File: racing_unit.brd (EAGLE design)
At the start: 81 x 80 mm, 55 parts, among them IC1 78L05Z, IC2 78L05Z, IC3 78L05Z, IC4 78L05Z, J1 J10MM, J2 J10MM, J3 J5MM, J4 J5MM, J5 J7MM, J7 J5MM, J8 J5MM, J9 J5MM, Q1 BDX54C, Q2 BDX54C, Q3 BDX54C, Q4 BDX54C

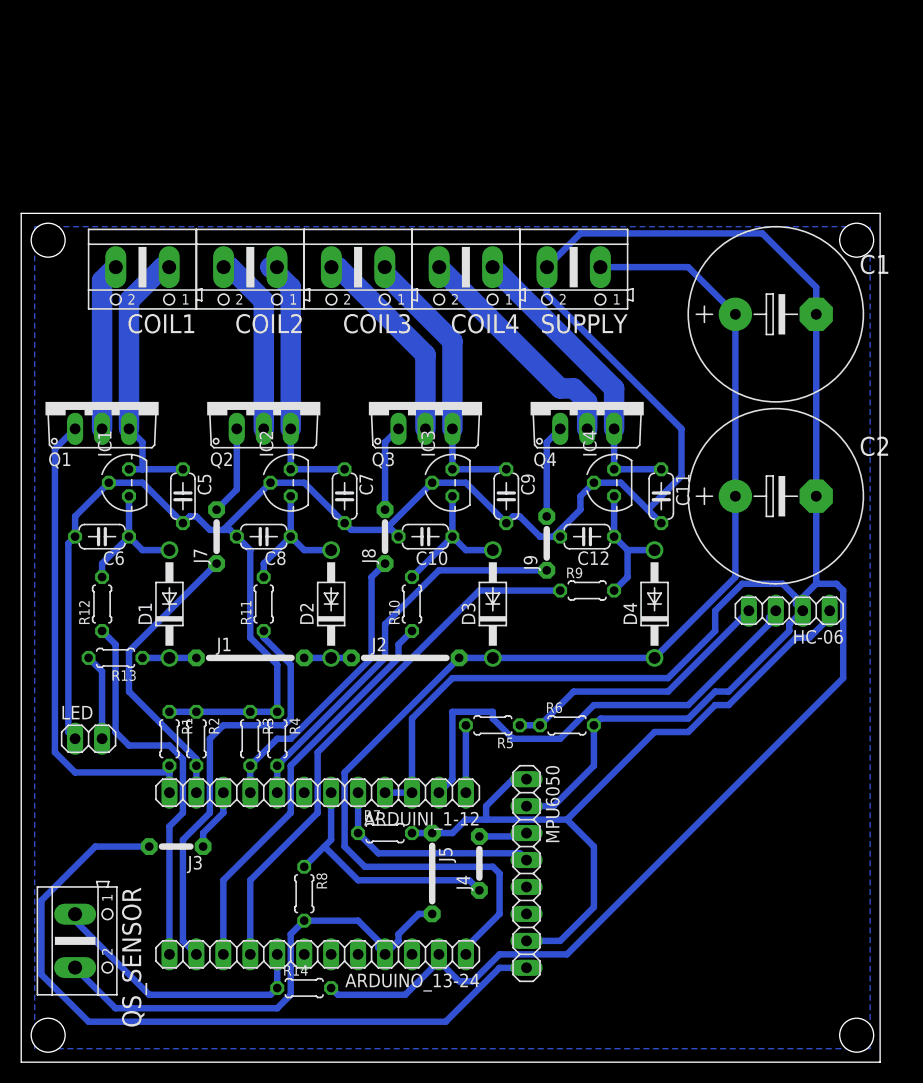
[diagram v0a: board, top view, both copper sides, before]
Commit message: updated pcb and schematic
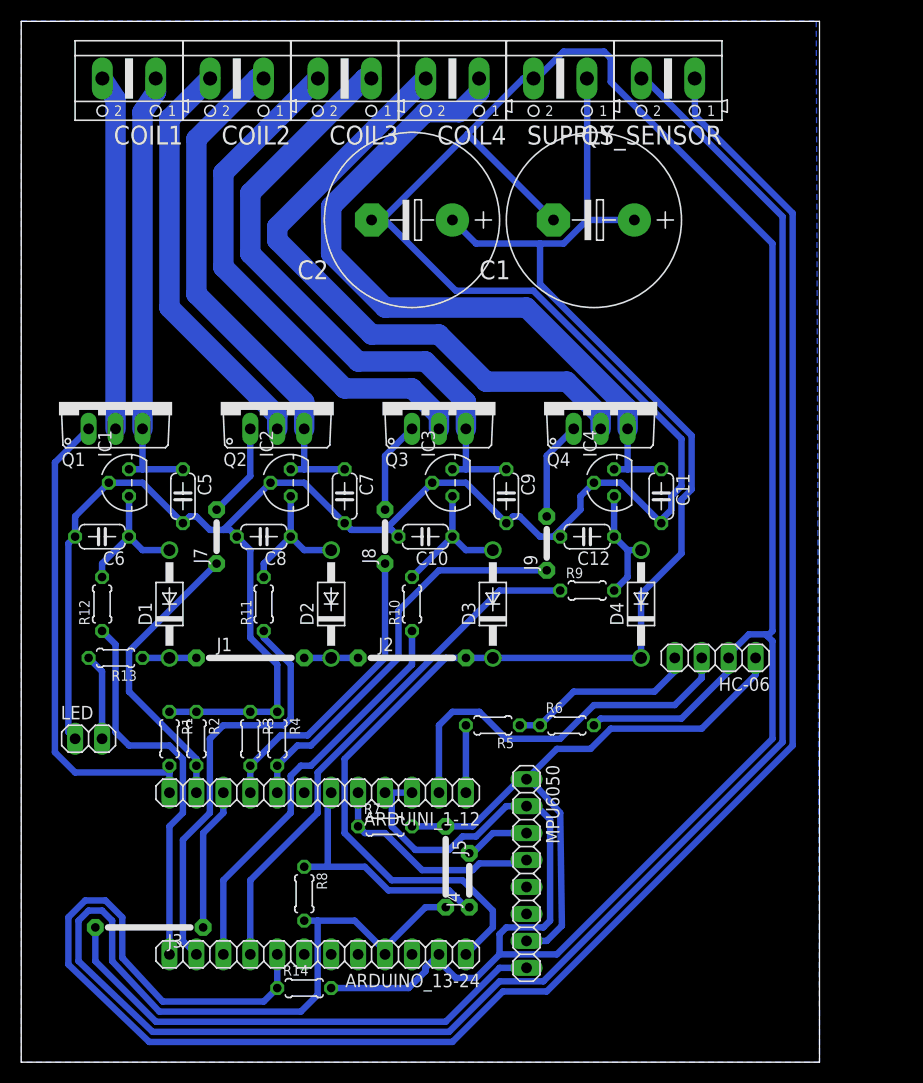
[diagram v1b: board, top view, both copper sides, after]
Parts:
- J3: value J5MM -> J10MM; device jumper:05 -> jumper:10
- moved QS_SENSOR 98.6 mm to (61.0, 92.7), turned to 180 degrees
- moved C2 43.1 mm to (36.8, 79.4), turned to 180 degrees
- moved C1 19.3 mm to (54.0, 79.4), turned to 180 degrees
- moved COIL1 17.8 mm to (10.2, 92.7)
- moved COIL2 17.8 mm to (20.3, 92.7)
- moved COIL3 17.8 mm to (30.5, 92.7)
- moved COIL4 17.8 mm to (40.6, 92.7)
- moved SUPPLY 17.8 mm to (50.8, 92.7)
- moved HC-06 8.28 mm to (65.4, 38.1)
- moved J3 8.03 mm to (12.1, 12.7)
- moved J4 1.85 mm to (42.2, 17.1)
- moved J5 1.42 mm to (40.0, 18.4)
- moved Q1 1.27 mm to (8.89, 62.2)
- moved Q2 1.27 mm to (24.1, 62.2)
- moved D4 1.27 mm to (58.4, 43.2)
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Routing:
- net N$18: track 45.7 -> 206.3 mm
- net N$16: track 26.0 -> 184.2 mm
- net N$4: track 28.3 -> 68.3 mm
- net N$9: track 21.8 -> 59.6 mm
- net N$3: track 26.8 -> 59.1 mm
- net N$10: track 19.3 -> 48.9 mm
- net N$19: track 114.7 -> 140.3 mm
- net N$2: track 25.5 -> 49.1 mm
- net N$11: track 17.2 -> 38.8 mm
- net N$29: track 68.9 -> 48.3 mm
- net GND: track 379.1 -> 398.7 mm
- net N$12: track 15.8 -> 33.4 mm
- net N$1: track 26.6 -> 42.3 mm
- net N$5: track 71.5 -> 59.0 mm
- net N$6: track 45.4 -> 37.0 mm
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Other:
- board size 81 x 80 mm -> 75.2 x 98.1 mm
- board text added: "Racing Unit"
